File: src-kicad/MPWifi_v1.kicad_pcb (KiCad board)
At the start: 2 copper layers, 16 parts, among them CON1 Micro_SD_Card, M1 ESP8266-12E, P1 CONN_01X04, P2 Flash, Q1 BSS138, Q2 BSS138, U1 MCP1703T-3302E/CB

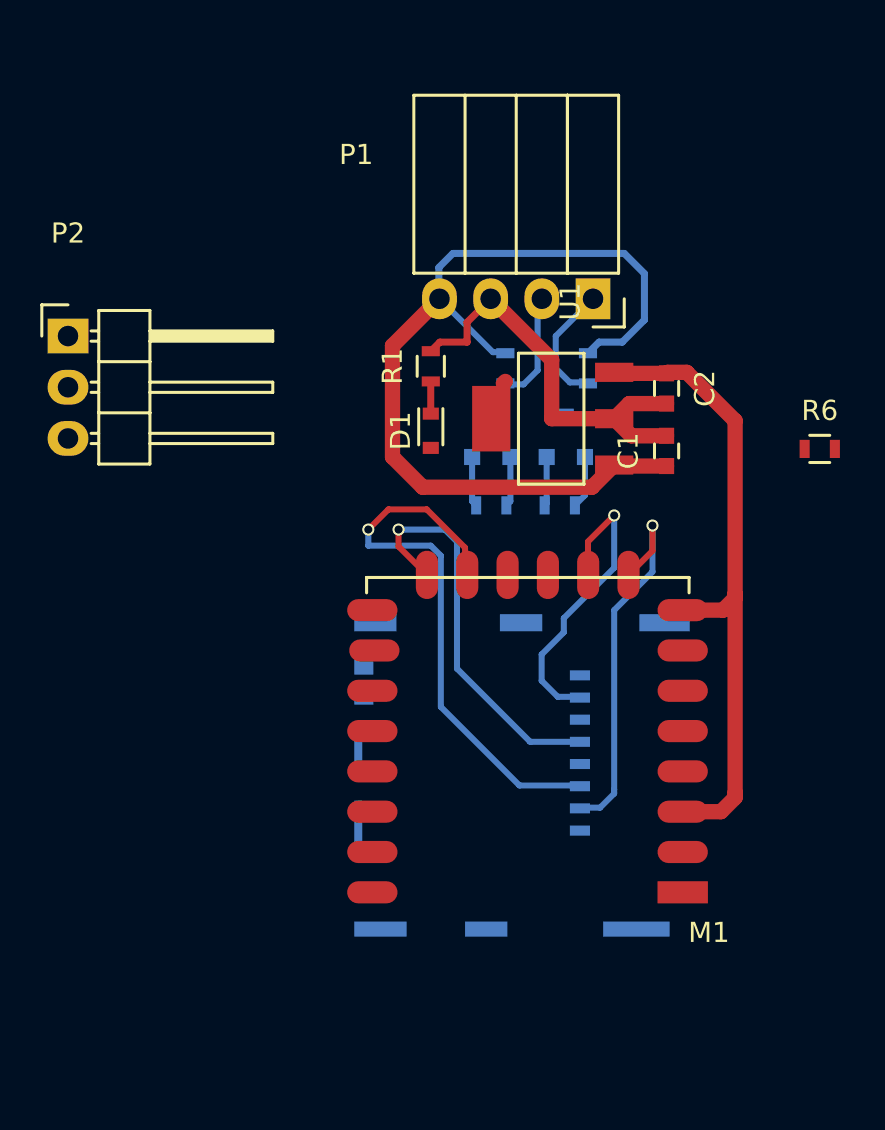
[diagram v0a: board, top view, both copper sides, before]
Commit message: Board v1.0 and BOM
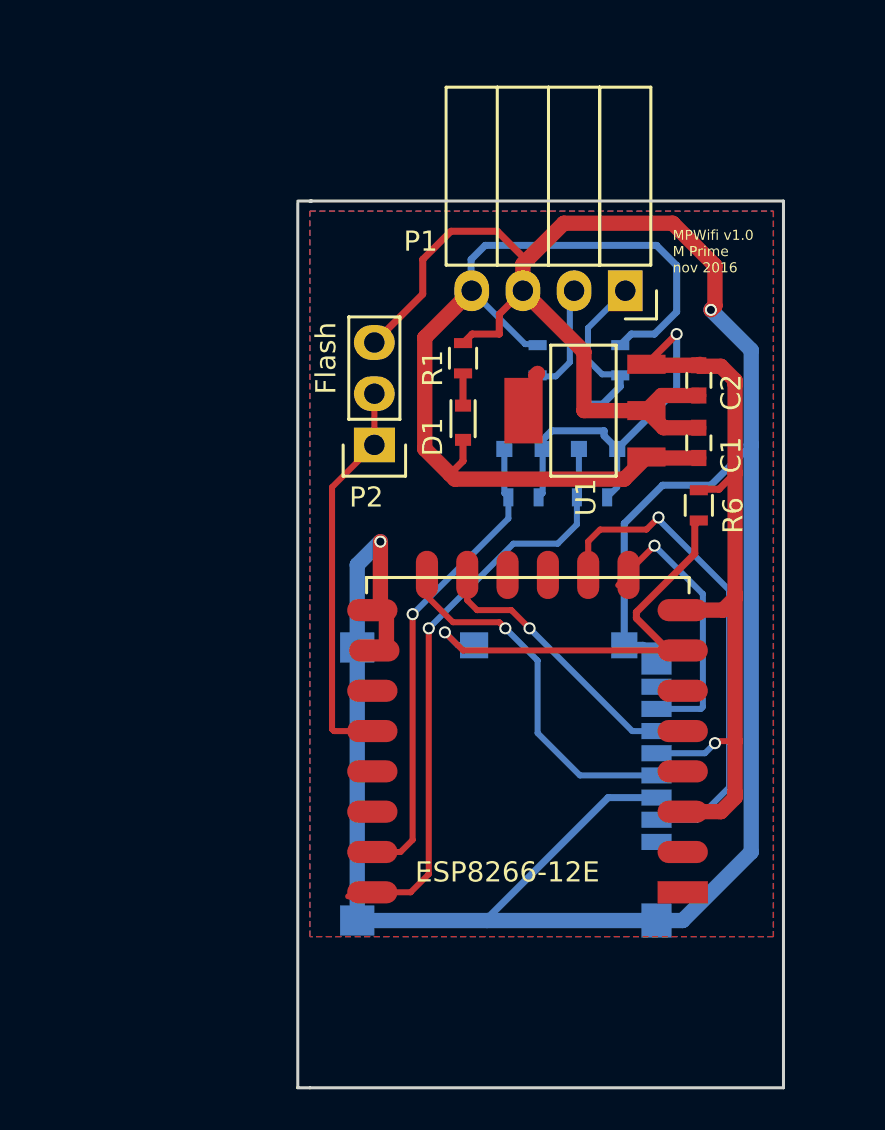
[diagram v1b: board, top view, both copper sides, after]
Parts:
- P2: footprint Pin_Headers:Pin_Header_Angled_1x03 -> Pin_Headers:Pin_Header_Straight_1x03
- moved CON1 21.5 mm to (149.0, 80.9), turned to 270 degrees
- moved P2 16.1 mm to (150.7, 70.1), turned to 180 degrees
- moved R6 6.62 mm to (166.8, 73.1), turned to 270 degrees
- moved C1 1.65 mm to (166.8, 70.0)
- moved Q1 1.65 mm to (161.8, 69.3)
- moved C2 1.65 mm to (166.8, 66.9)
- moved R3 1.65 mm to (158.8, 65.9)
- moved D1 1.65 mm to (155.1, 69.0)
- moved Q2 1.65 mm to (158.1, 69.3)
- moved R1 1.65 mm to (155.1, 65.8)
- moved P1 1.65 mm to (163.2, 62.5)
- moved R2 1.65 mm to (162.9, 65.9)
- moved R4 1.65 mm to (161.5, 72.7)
- moved R5 1.65 mm to (158.1, 72.7)
- moved U1 1.65 mm to (164.2, 68.4)
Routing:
- net GND: track 21.2 -> 149.9 mm, vias 0 -> 2
- net Net-(M1-Pad16): track 2.44 -> 30.1 mm, vias 0 -> 1
- net /DETECT_SWITCH: track 0.00 -> 21.6 mm, vias 0 -> 1
- net Net-(M1-Pad15): track 2.48 -> 23.1 mm, vias 0 -> 1
- net Net-(M1-Pad12): track 0.00 -> 20.3 mm
- net +3V3: track 38.3 -> 58.5 mm, vias 0 -> 2
- net /MOSI: track 28.0 -> 13.8 mm
- net /MISO: track 15.5 -> 25.1 mm
- net /CS: track 19.0 -> 14.0 mm
- net /TX: track 6.48 -> 8.59 mm
- net VCC: track 46.3 -> 48.2 mm
- net /SCLK: track 19.9 -> 18.5 mm
- added copper zone on B.Cu, net GND
- added copper zone on F.Cu, net GND
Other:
- board outline added: 24.1 x 44 mm
- net class Default: clearance 0.2 -> 0.1492
- rule trace_clearance: 0.2 -> 0.1492
- board text added: "MPWifi v1.0 M Prime nov 2016"

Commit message: v1.0 PCB
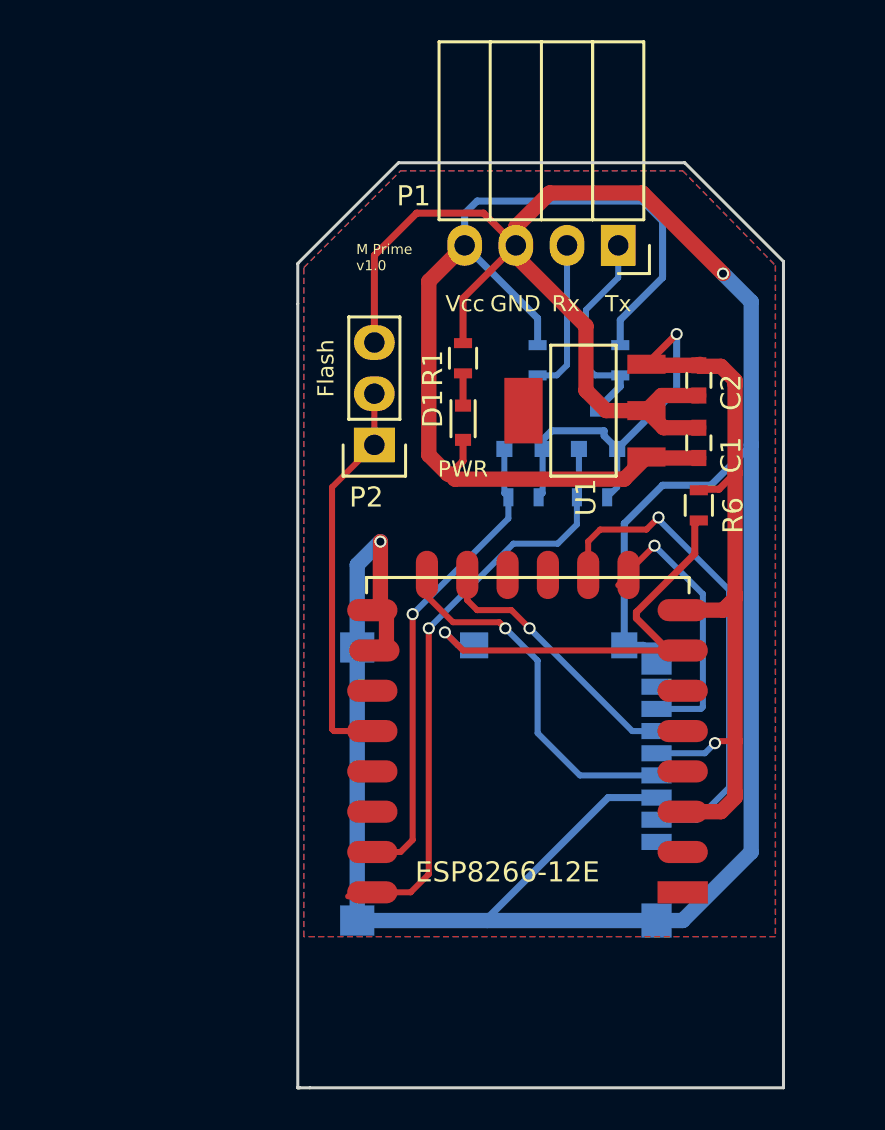
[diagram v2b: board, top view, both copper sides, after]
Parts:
- moved P1 2.28 mm to (162.8, 60.2)
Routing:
- net VCC: track 48.2 -> 53.1 mm
- net GND: track 149.9 -> 152.4 mm
- net /TX: track 8.59 -> 10.7 mm
- net /RX: track 7.49 -> 9.62 mm
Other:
- board size 24.1 x 44 mm -> 24.1 x 45.9 mm
- board text added: "GND"
- board text added: "M Prime v1.0"
- board text added: "PWR"
- board text added: "Rx"
- board text added: "Tx"
- board text added: "Vcc"
- board text removed: "MPWifi v1.0 M Prime nov 2016"
